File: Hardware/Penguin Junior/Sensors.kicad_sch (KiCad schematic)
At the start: 5 parts, among them U2 MS5611-01BA, U3 BMI088

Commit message: Updated project
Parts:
- C14, C15, C16: footprint Capacitor_SMD:C_0603_1608Metric -> Capacitor_SMD:C_0402_1005Metric
- U2: footprint Package_LGA:LGA-8_3x5mm_P1.25mm -> user_lib:LGA-8_3x5mm_P1.25mm_handsolder
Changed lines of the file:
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@@
       (effects (font (size 1.27 1.27)))
     )
-    (property "Footprint" "Capacitor_SMD:C_0603_1608Metric" (at 208.28 89.8398 0)
+    (property "Footprint" "Capacitor_SMD:C_0402_1005Metric" (at 208.28 89.8398 0)
       (effects (font (size 1.27 1.27)) hide)
     )
@@
       (effects (font (size 1.27 1.27)))
     )
-    (property "Footprint" "Capacitor_SMD:C_0603_1608Metric" (at 218.44 89.8398 0)
+    (property "Footprint" "Capacitor_SMD:C_0402_1005Metric" (at 218.44 89.8398 0)
       (effects (font (size 1.27 1.27)) hide)
     )
@@
       (effects (font (size 1.27 1.27)) (justify left))
     )
-    (property "Footprint" "Capacitor_SMD:C_0603_1608Metric" (at 205.4352 43.815 0)
+    (property "Footprint" "Capacitor_SMD:C_0402_1005Metric" (at 205.4352 43.815 0)
       (effects (font (size 1.27 1.27)) hide)
     )
@@
       (effects (font (size 1.27 1.27)) (justify left))
     )
-    (property "Footprint" "Package_LGA:LGA-8_3x5mm_P1.25mm" (at 189.865 40.005 0)
+    (property "Footprint" "user_lib:LGA-8_3x5mm_P1.25mm_handsolder" (at 189.865 40.005 0)
       (effects (font (size 1.27 1.27)) hide)
     )

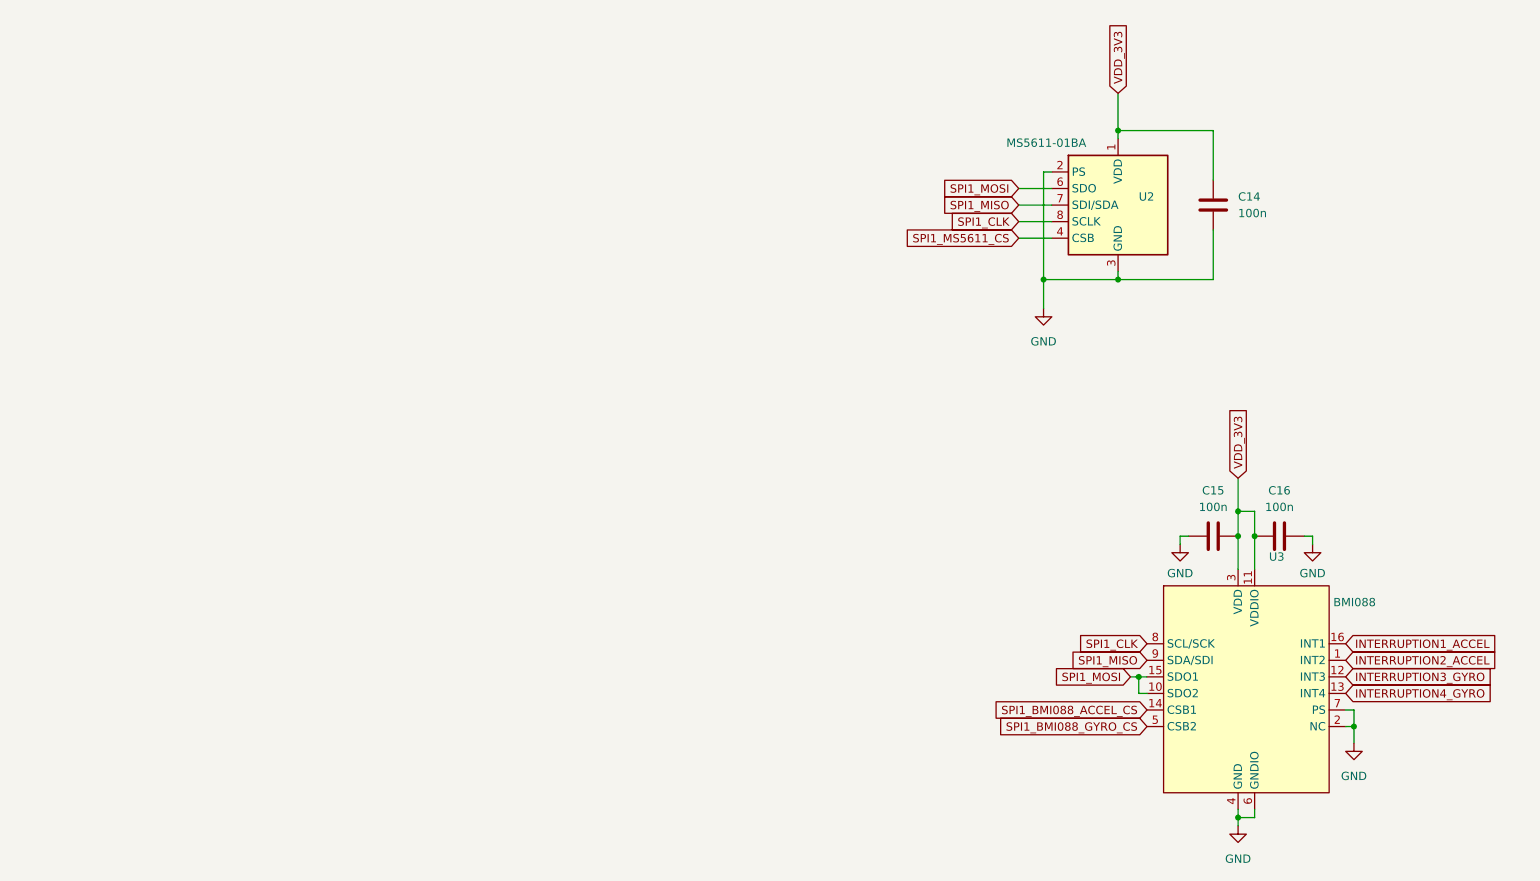
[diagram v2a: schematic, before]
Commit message: Penguin Junior 1.1 release
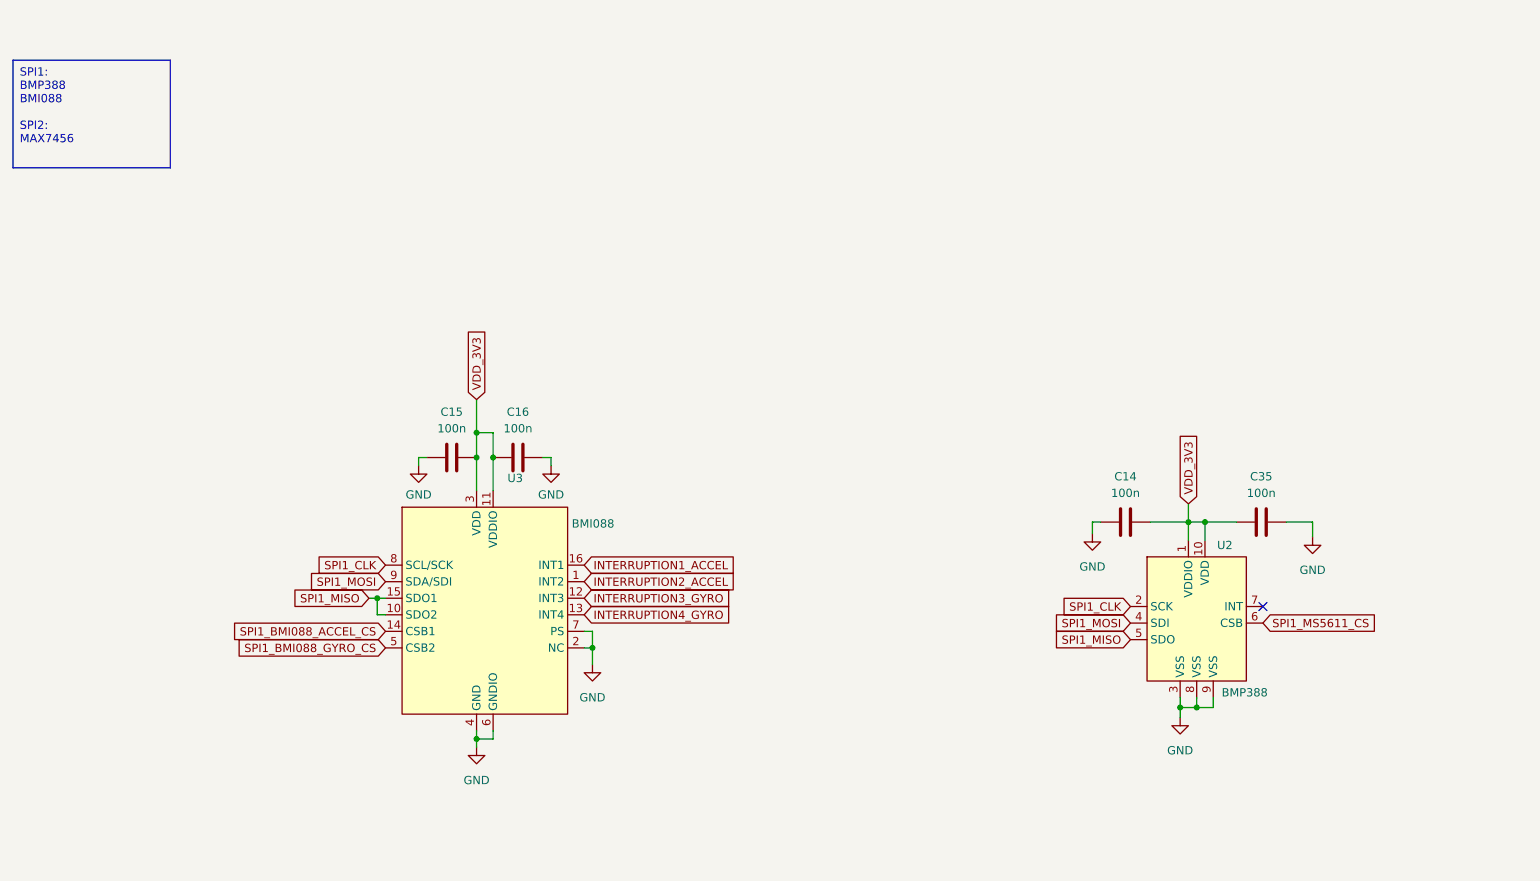
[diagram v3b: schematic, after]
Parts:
- removed U2: MS5611-01BA, user_lib:LGA-8_3x5mm_P1.25mm_handsolder, symbol Sensor_Pressure:MS5611-01BA
- added C35: 100n, Capacitor_SMD:C_0402_1005Metric, symbol Device:C
- added U2: BMP388, user_lib:LGA-10_2x2x0.75mm, symbol user_lib:BMP388
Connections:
- net GND: now also C14.1, C35.2, U2.3 (VSS), U2.8 (VSS), U2.9 (VSS); no longer C14.2
- net SPI1_CLK: now also U2.2 (SCK)
- net SPI1_MISO: now also U3.10 (SDO2), U3.15 (SDO1), U2.5 (SDO); no longer U3.9 (SDA/SDI)
- net SPI1_MOSI: now also U3.9 (SDA/SDI), U2.4 (SDI); no longer U3.10 (SDO2), U3.15 (SDO1)
- net SPI1_MS5611_CS: now also U2.6 (CSB)
- net VDD_3V3: now also C14.2, C35.1, U2.1 (VDDIO), U2.10 (VDD); no longer C14.1
- no-connect marks 0 -> 1
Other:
- moved on the sheet: C15, C16, U3
